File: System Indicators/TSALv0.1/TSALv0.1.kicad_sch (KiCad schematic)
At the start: 3 parts, among them U1 LM311, U2 NA555P, U3 4N35

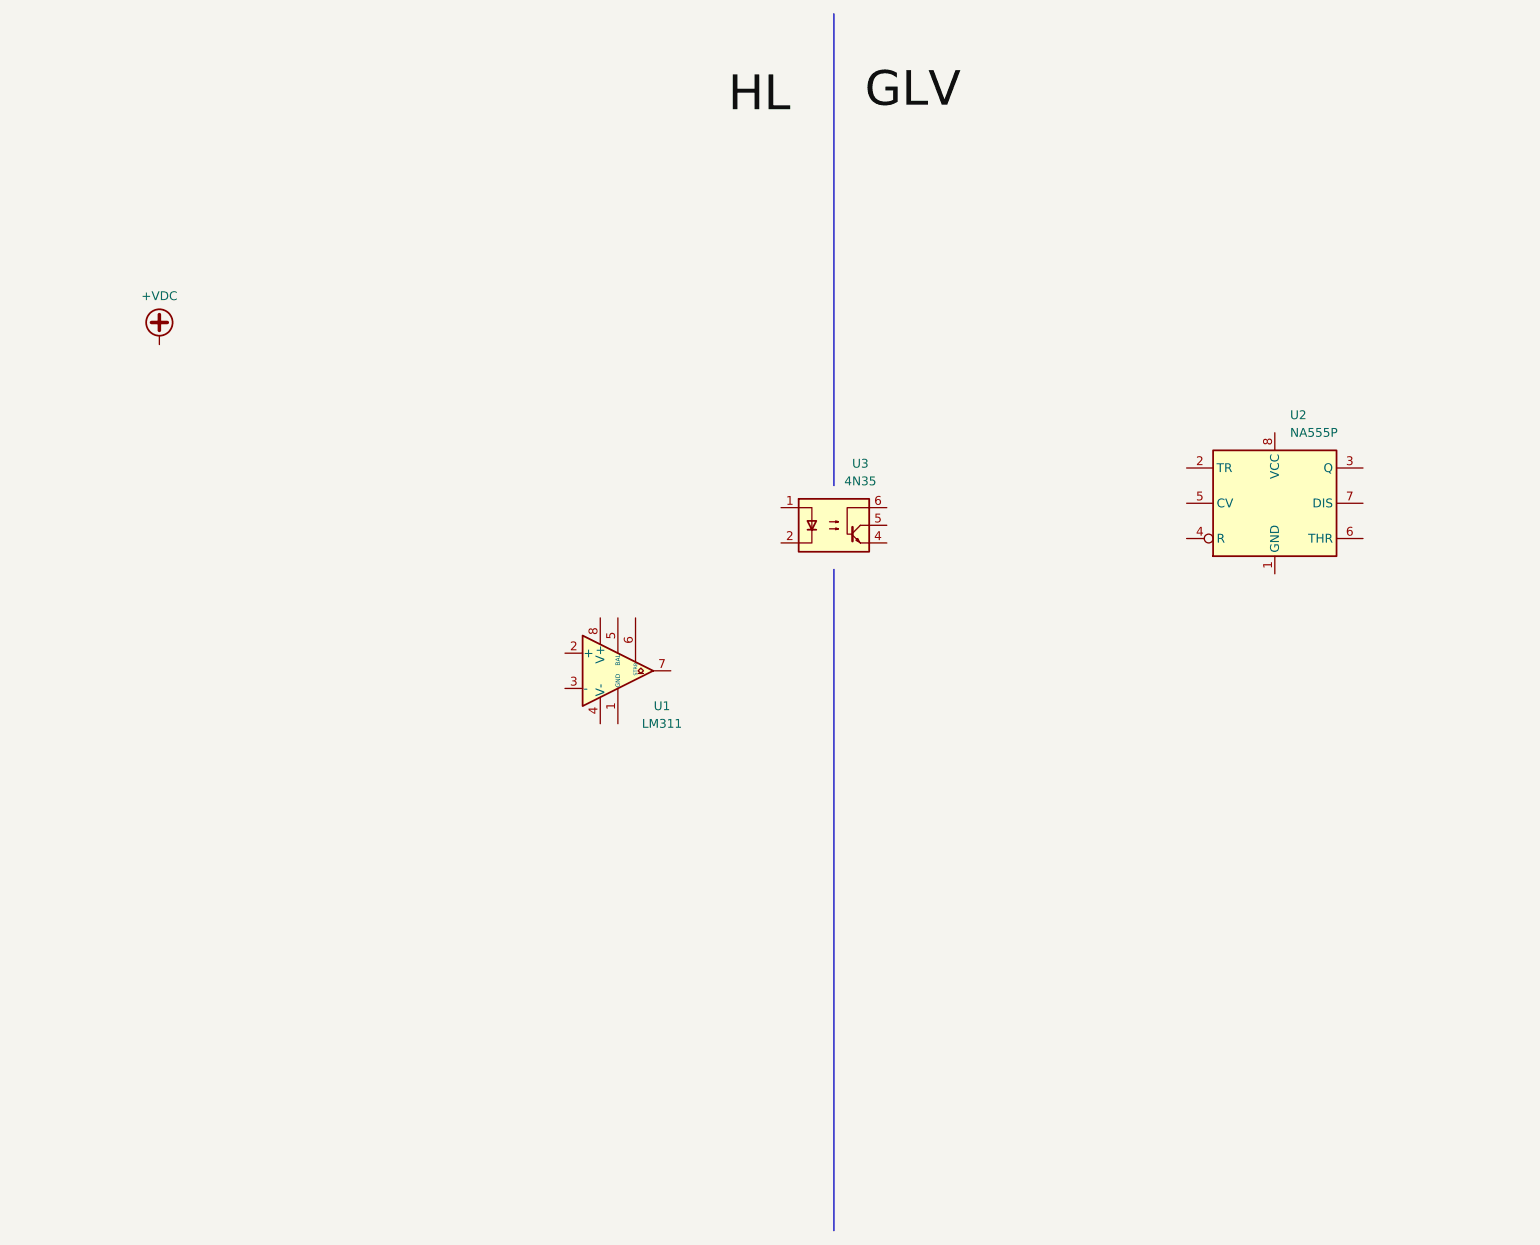
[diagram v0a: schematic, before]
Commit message: Updated Schematic
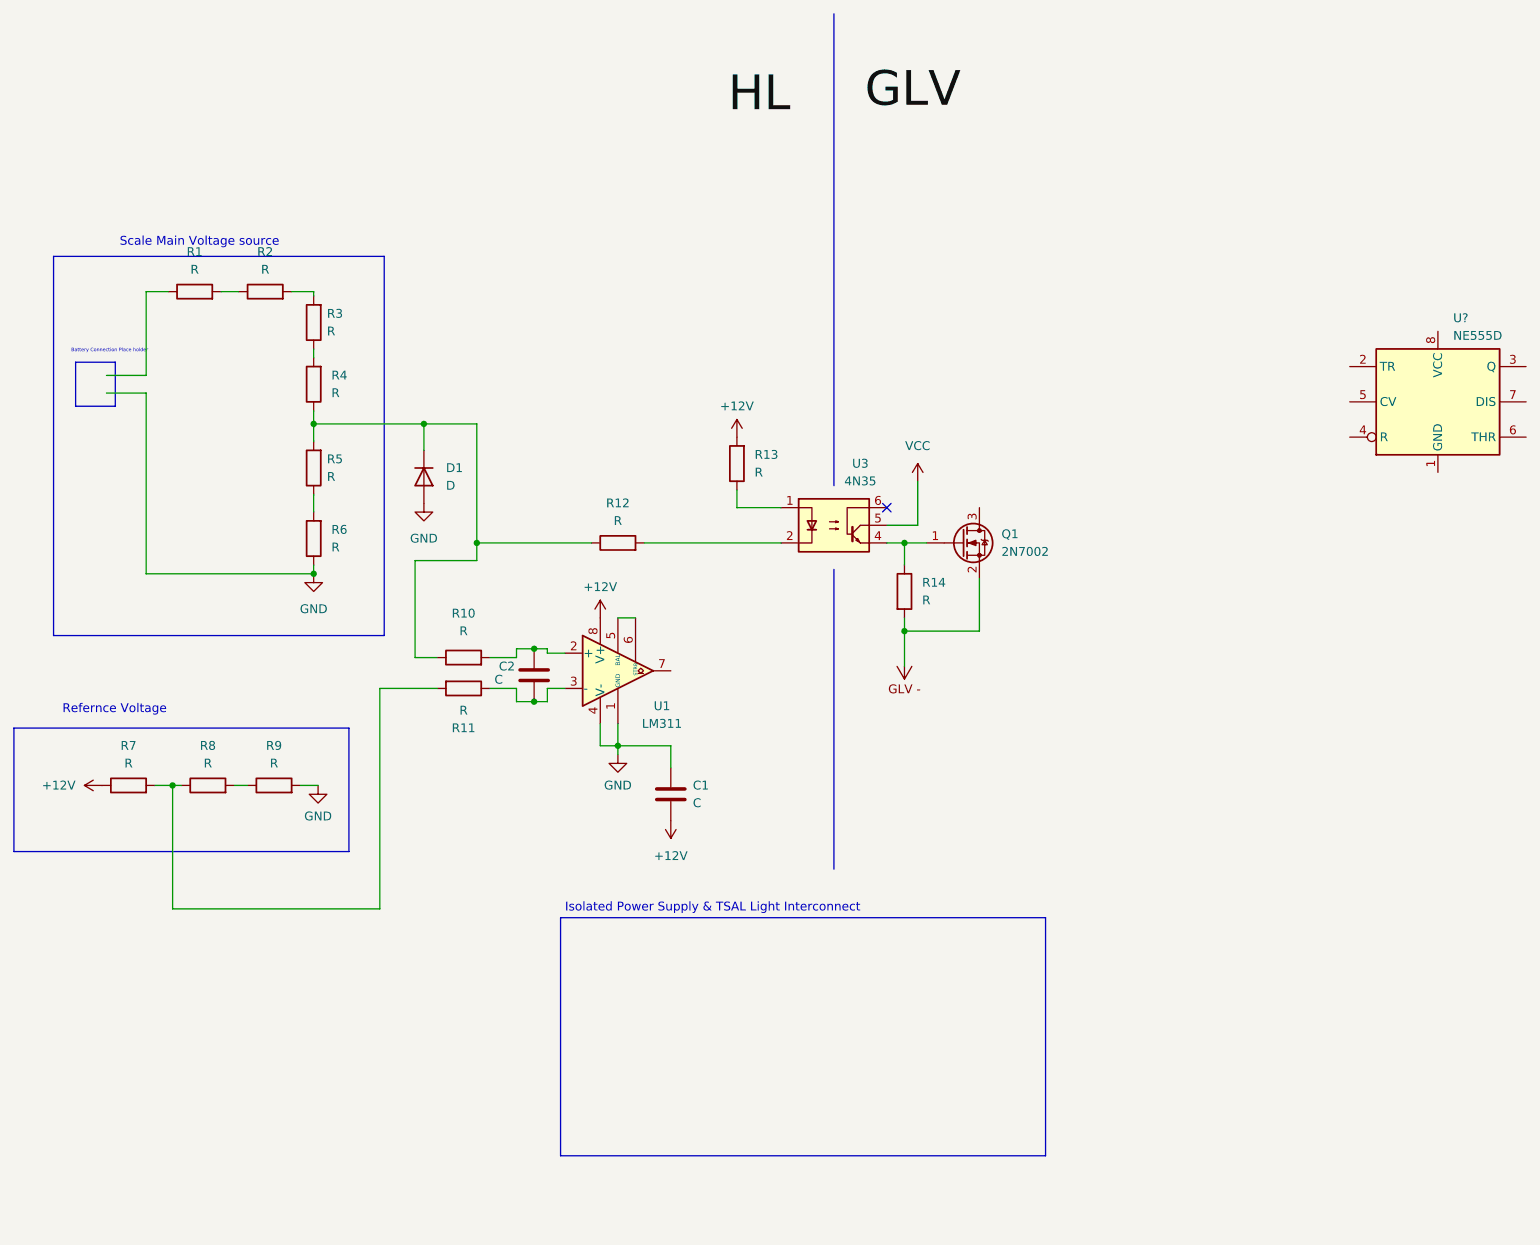
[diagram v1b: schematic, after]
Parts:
- added C1, C2: C, symbol Device:C
- added D1: D, symbol Device:D
- added Q1: 2N7002, Package_TO_SOT_SMD:SOT-23, symbol Transistor_FET:2N7002
- added R1, R10, R11, R12, R13, R14, R2, R3, R4, R5, R6, R7, R8, R9: R, symbol Device:R
- U?: renamed from U2; value NA555P -> NE555D; footprint Package_DIP:DIP-8_W7.62mm -> Package_SO:SOIC-8_3.9x4.9mm_P1.27mm; symbol Timer:NA555P -> Timer:NE555D
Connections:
- net at U3.1: now also R13.1
- net at U3.2: now also R12.2
- net at U3.4: now also Q1.1 (G), R14.1
- net VCC: now reaches U3.5
- net GND: now reaches U1.1 (GND)
- net GND: now also U1.4 (V-), C1.1, D1.2 (A), R6.1, R9.2
- net at U1.2 (+): now also C2.1, R10.2
- net at U1.3 (-): now also C2.2, R11.1
- net at U1.5 (BAL): now also U1.6 (STRB)
- net +12V: now reaches U1.8 (V+)
- net +12V: now also C1.2, R13.2, R7.1
- new net: R1.2, R2.1
- new net: R2.2, R3.2
- new net: D1.1 (K), R10.1, R12.1, R4.1, R5.2
- new net: R3.1, R4.2
- new net: R8.2, R9.1
- new net: R11.2, R7.2, R8.1
- new net: R5.1, R6.2
- new net -: Q1.2 (S), R14.2
- no-connect marks 0 -> 1
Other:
- note added: "Battery Connection Place holder"
- note added: "Isolated Power Supply & TSAL Light Interconnect"
- note added: "Refernce Voltage"
- note added: "Scale Main Voltage source"
- moved on the sheet: U?
